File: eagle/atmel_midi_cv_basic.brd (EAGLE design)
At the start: 101 x 80.8 mm, 46 parts, among them IC1 TL072P, IC2 TL072P, U1 ATMEGA328P_PDIP

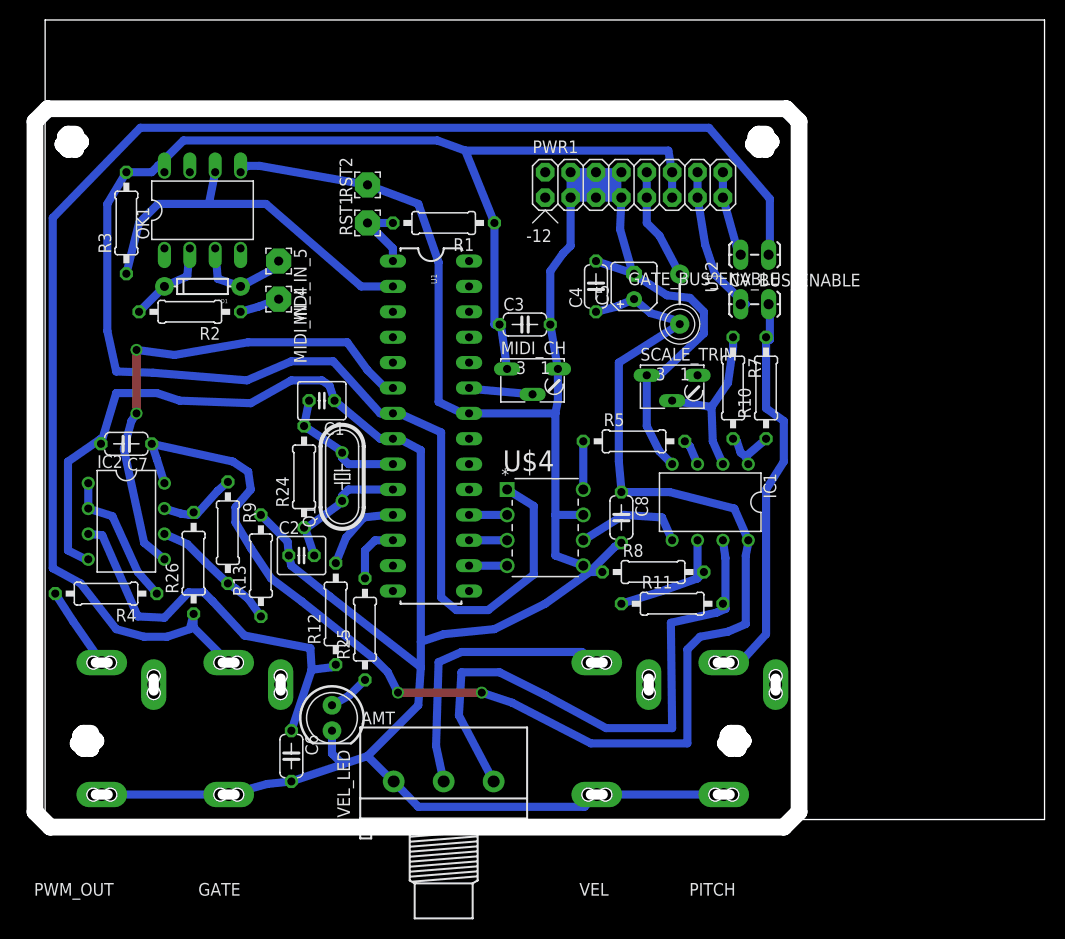
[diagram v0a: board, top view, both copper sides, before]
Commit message: cleaned up some routes
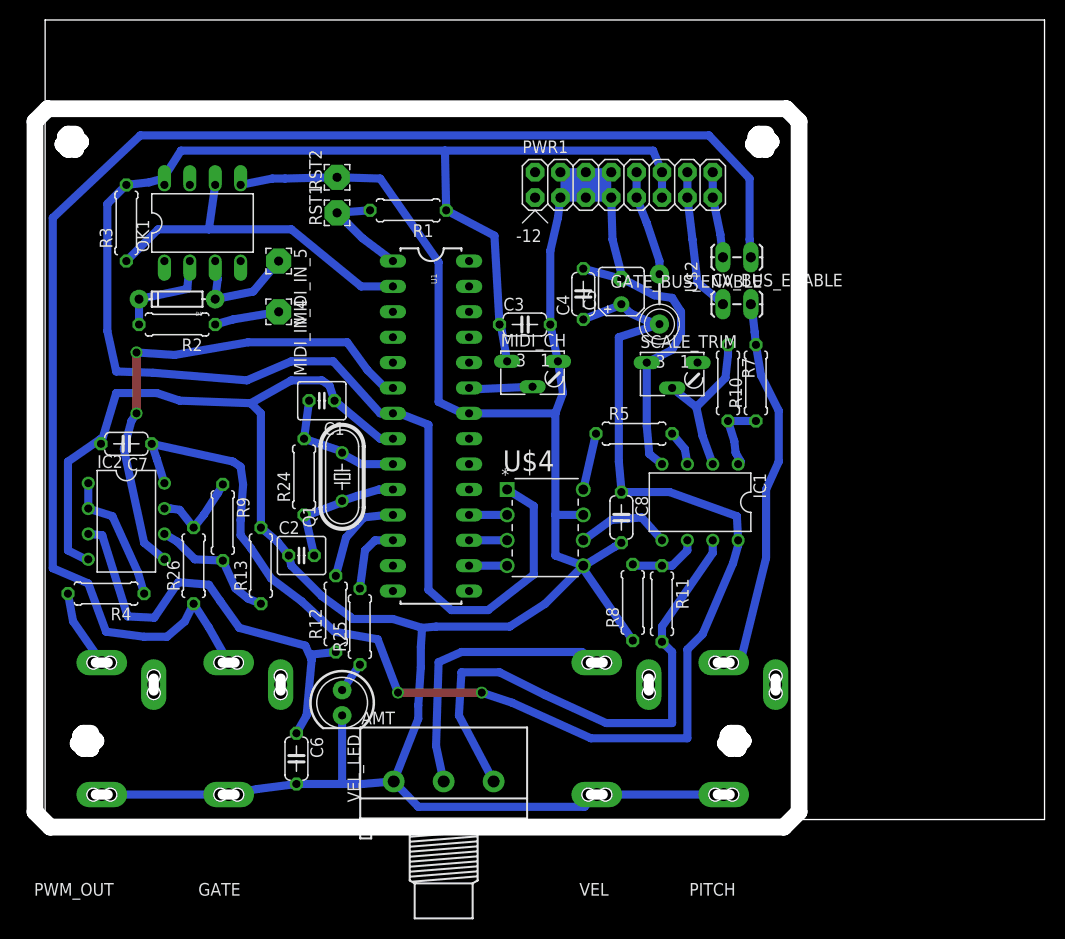
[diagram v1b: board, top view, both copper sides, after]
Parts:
- R1, R10, R11, R12, R13, R2, R24, R25, R26, R3, R4, R5, R7, R8, R9: device rcl:0207/10 -> rcl:0207/7
- moved R1 3.78 mm to (36.3, 61.0)
- moved R8 3.66 mm to (58.8, 21.7), turned to 90 degrees
- moved RST1 3.21 mm to (29.2, 60.7)
- moved RST2 3.14 mm to (29.2, 64.3)
- moved D1 2.84 mm to (13.2, 52.1)
- moved U$2 2.03 mm to (61.5, 52.1)
- moved VEL_LED 1.83 mm to (29.7, 11.7)
- moved GATE_BUS_ENABLE 1.80 mm to (70.5, 56.3)
- moved R2 1.80 mm to (13.2, 49.5)
- moved CV_BUS_ENABLE 1.78 mm to (67.9, 51.6)
- moved C4 1.48 mm to (53.8, 52.6)
- moved C5 1.37 mm to (57.7, 52.8)
- moved MIDI_IN_4 1.27 mm to (23.4, 50.8)
- moved OK1 1.27 mm to (15.7, 59.7)
- moved SCALE_TRIM 1.27 mm to (62.7, 45.7)
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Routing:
- net N$29: track 346.8 -> 339.8 mm
- net N$32: track 0.00 -> 6.35 mm
- net N$13: track 12.7 -> 7.16 mm
- net +12V: track 142.9 -> 137.6 mm
- net N$9: track 42.8 -> 38.7 mm
- net GND: track 3.72 -> 0.00 mm
- net N$17: track 57.9 -> 54.3 mm
- net N$43: track 7.40 -> 10.7 mm
- net N$30: track 37.7 -> 34.5 mm
- net N$28: track 41.7 -> 44.2 mm
- net N$8: track 4.02 -> 6.48 mm
- net N$27: track 5.80 -> 7.46 mm
- net N$14: track 11.1 -> 9.57 mm
- net N$3: track 10.3 -> 11.7 mm
- net N$7: track 8.90 -> 10.3 mm
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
